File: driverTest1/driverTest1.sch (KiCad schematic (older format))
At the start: 50 parts, among them J1 LED_OUT, J2 INPUT, Q1 2N7002, Q2 2N7002, U1 TPS63020, U2 TPH2504-SR, U3 XC6206P332MR

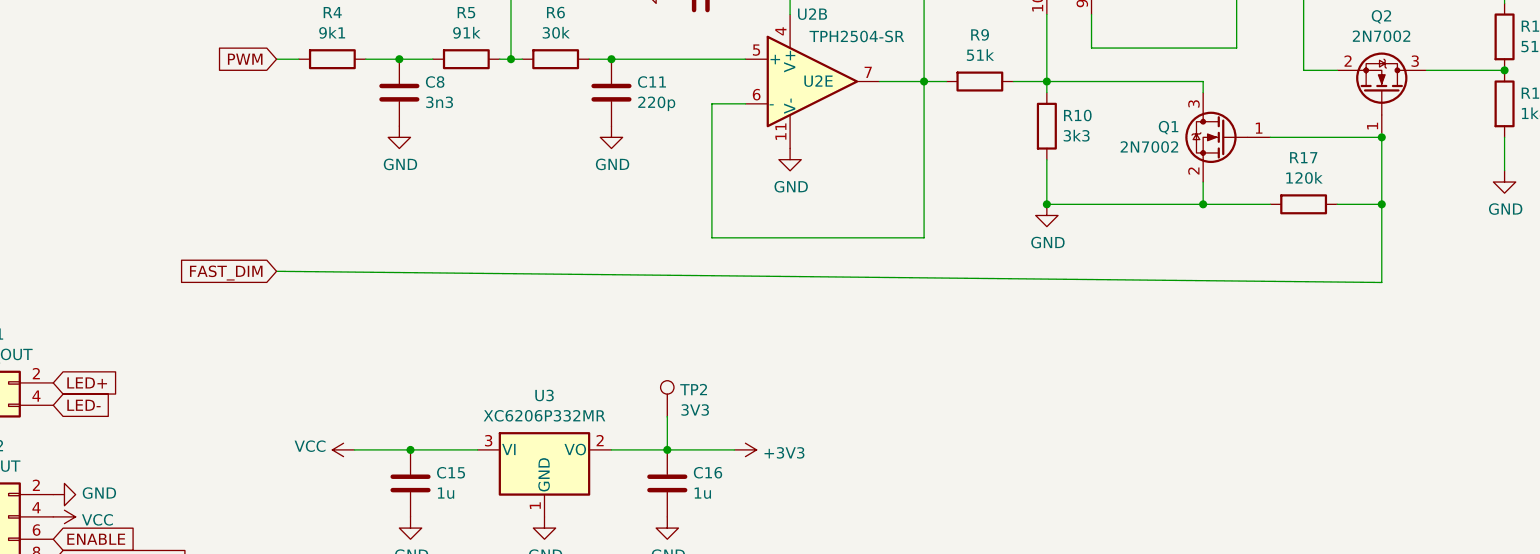
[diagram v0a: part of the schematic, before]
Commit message: Tweak assembly data
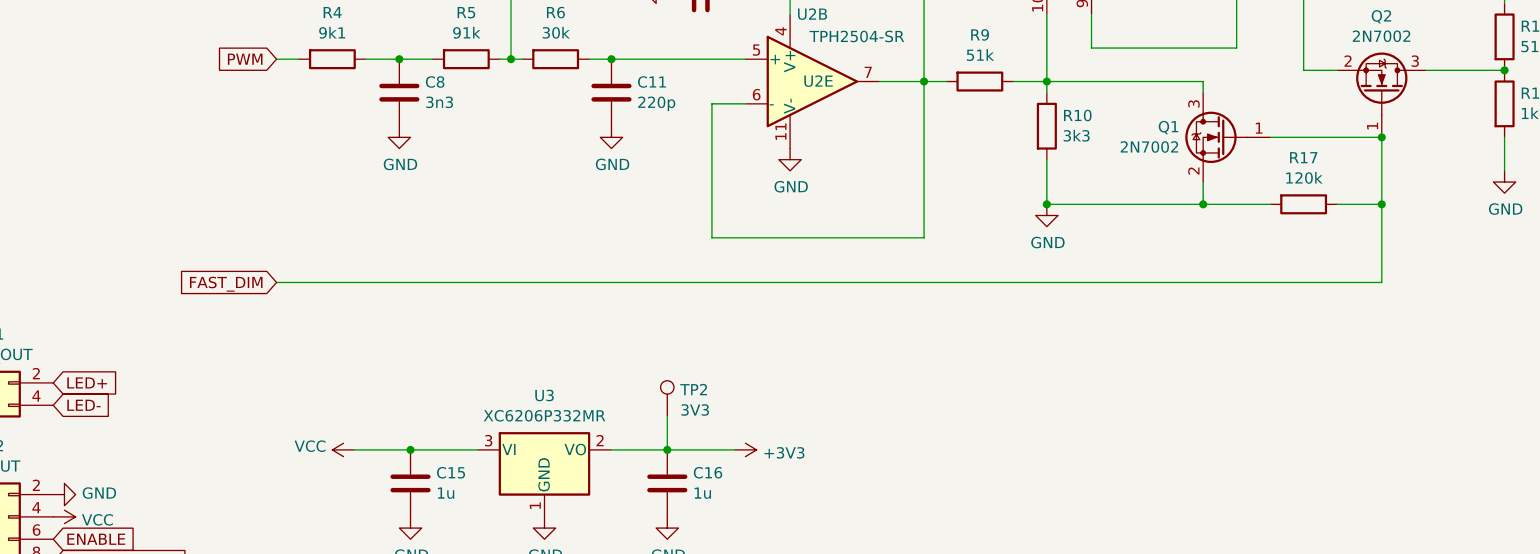
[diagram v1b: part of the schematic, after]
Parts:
- Q1, Q2, U3: JLCPCB_CORRECTION (none) -> 0;0;180
- U2: JLCPCB_CORRECTION (none) -> 0;0;-90
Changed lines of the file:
@@
 F 3 "https://www.torexsemi.com/file/xc6206/XC6206.pdf" H 4650 6550 50  0001 C CNN
 F 4 "C5446" H 4650 6550 50  0001 C CNN "LCSC"
+F 5 "0;0;180" H 4650 6550 50  0001 C CNN "JLCPCB_CORRECTION"
 	1    4650 6550
 	1    0    0    -1
@@
 F 3 "http://www.ti.com/lit/ds/symlink/lm2902-n.pdf" H 6150 3400 50  0001 C CNN
 F 4 "C115918" H 6100 3200 50  0001 C CNN "LCSC"
+F 5 "0;0;-90" H 6100 3200 50  0001 C CNN "JLCPCB_CORRECTION"
 	1    6100 3200
 	-1   0    0    -1
@@
 F 3 "http://www.ti.com/lit/ds/symlink/lm2902-n.pdf" H 5900 5100 50  0001 C CNN
 F 4 "C115918" H 5850 4900 50  0001 C CNN "LCSC"
+F 5 "0;0;-90" H 5850 4900 50  0001 C CNN "JLCPCB_CORRECTION"
 	2    5850 4900
 	1    0    0    -1
@@
 F 3 "http://www.ti.com/lit/ds/symlink/lm2902-n.pdf" H 7050 4500 50  0001 C CNN
 F 4 "C115918" H 7000 4300 50  0001 C CNN "LCSC"
+F 5 "0;0;-90" H 7000 4300 50  0001 C CNN "JLCPCB_CORRECTION"
 	3    7000 4300
 	0    -1   -1   0
@@
 F 3 "http://www.ti.com/lit/ds/symlink/lm2902-n.pdf" H 5900 5100 50  0001 C CNN
 F 4 "C115918" H 5850 4900 50  0001 C CNN "LCSC"
+F 5 "0;0;-90" H 5850 4900 50  0001 C CNN "JLCPCB_CORRECTION"
 	5    5850 4900
 	1    0    0    -1
@@
 F 3 "https://www.fairchildsemi.com/datasheets/2N/2N7002.pdf" H 7700 5150 50  0001 L CNN
 F 4 "C8545" H 7700 5150 50  0001 C CNN "LCSC"
+F 5 "0;0;180" H 7700 5150 50  0001 C CNN "JLCPCB_CORRECTION"
 	1    7700 5150
 	-1   0    0    -1
@@
 F 3 "https://www.fairchildsemi.com/datasheets/2N/2N7002.pdf" H 8400 4950 50  0001 L CNN
 F 4 "C8545" H 8400 4950 50  0001 C CNN "LCSC"
+F 5 "0;0;180" H 8400 4950 50  0001 C CNN "JLCPCB_CORRECTION"
 	1    8400 4950
 	0    1    -1   0
@@
 	8400 5450 8400 5800
 Wire Wire Line
-	8400 5800 3450 5750
+	8400 5800 3450 5800
 Connection ~ 8400 5450
-Text GLabel 3450 5750 0    50   Input ~ 0
+Text GLabel 3450 5800 0    50   Input ~ 0
 FAST_DIM
 Text GLabel 1950 7250 0    50   Input ~ 0
@@
 F 3 "http://www.ti.com/lit/ds/symlink/lm2902-n.pdf" H 7600 2950 50  0001 C CNN
 F 4 "C115918" H 7550 2750 50  0001 C CNN "LCSC"
+F 5 "0;0;-90" H 7550 2750 50  0001 C CNN "JLCPCB_CORRECTION"
 	4    7550 2750
 	0    -1   1    0
@@
 	1800 2350 3350 2350
 $Comp
-L power:+3.3V #PWR?
+L power:+3.3V #PWR0106
 U 1 1 5F85B2BF
 P 2300 2450
-F 0 "#PWR?" H 2300 2300 50  0001 C CNN
+F 0 "#PWR0106" H 2300 2300 50  0001 C CNN
 F 1 "+3.3V" H 2315 2623 50  0000 C CNN
 F 2 "" H 2300 2450 50  0001 C CNN
